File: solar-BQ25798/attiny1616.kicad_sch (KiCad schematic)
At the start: 14 parts, among them J1901 Conn_01x04, U1901 ATtiny1616-M

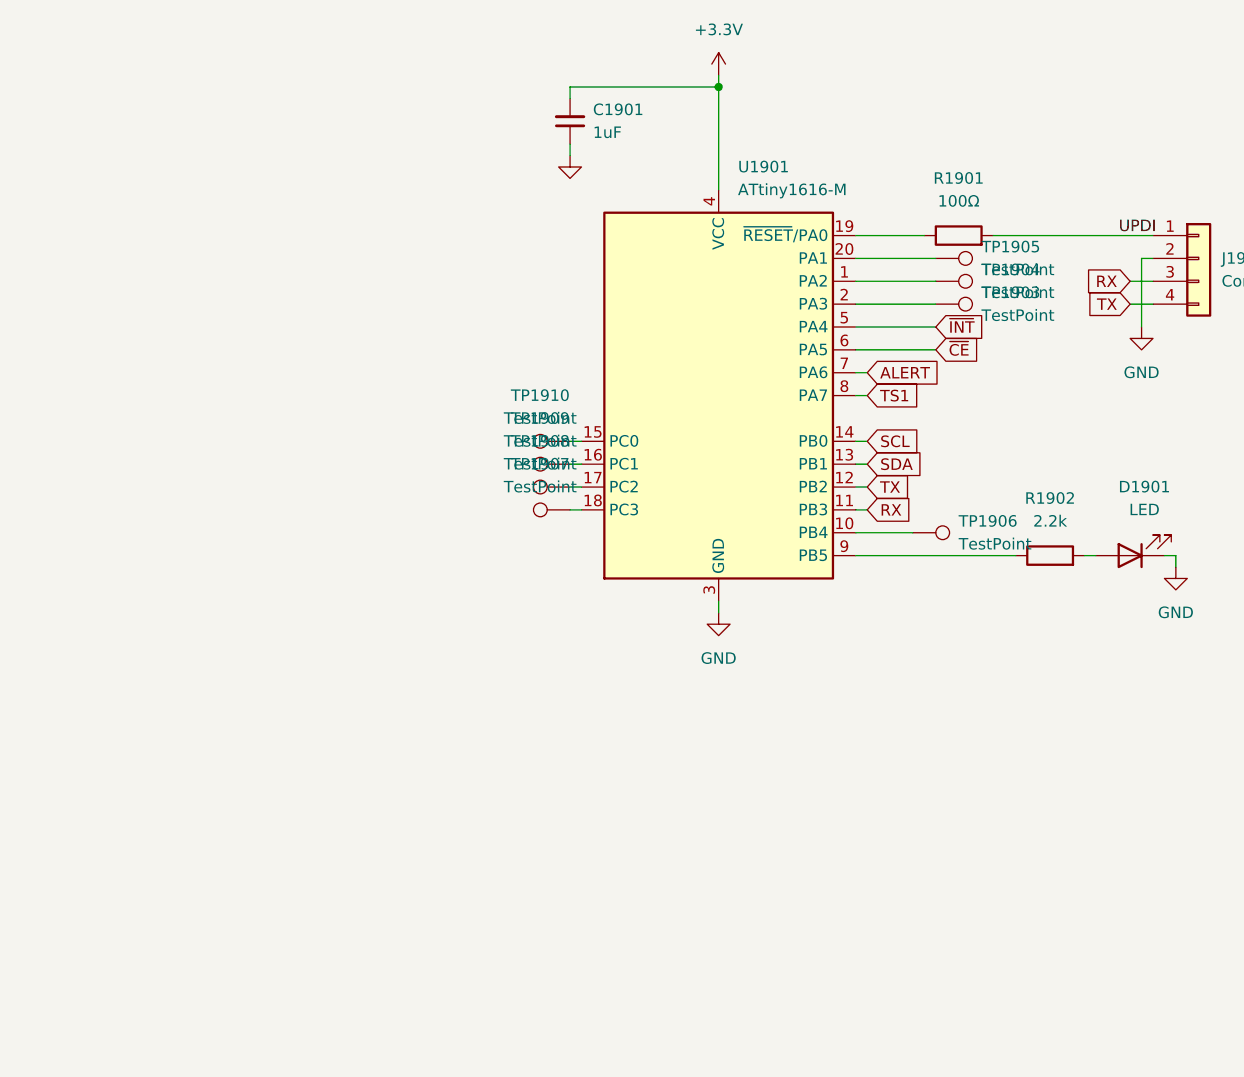
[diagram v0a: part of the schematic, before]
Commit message: BQ25798 WIP
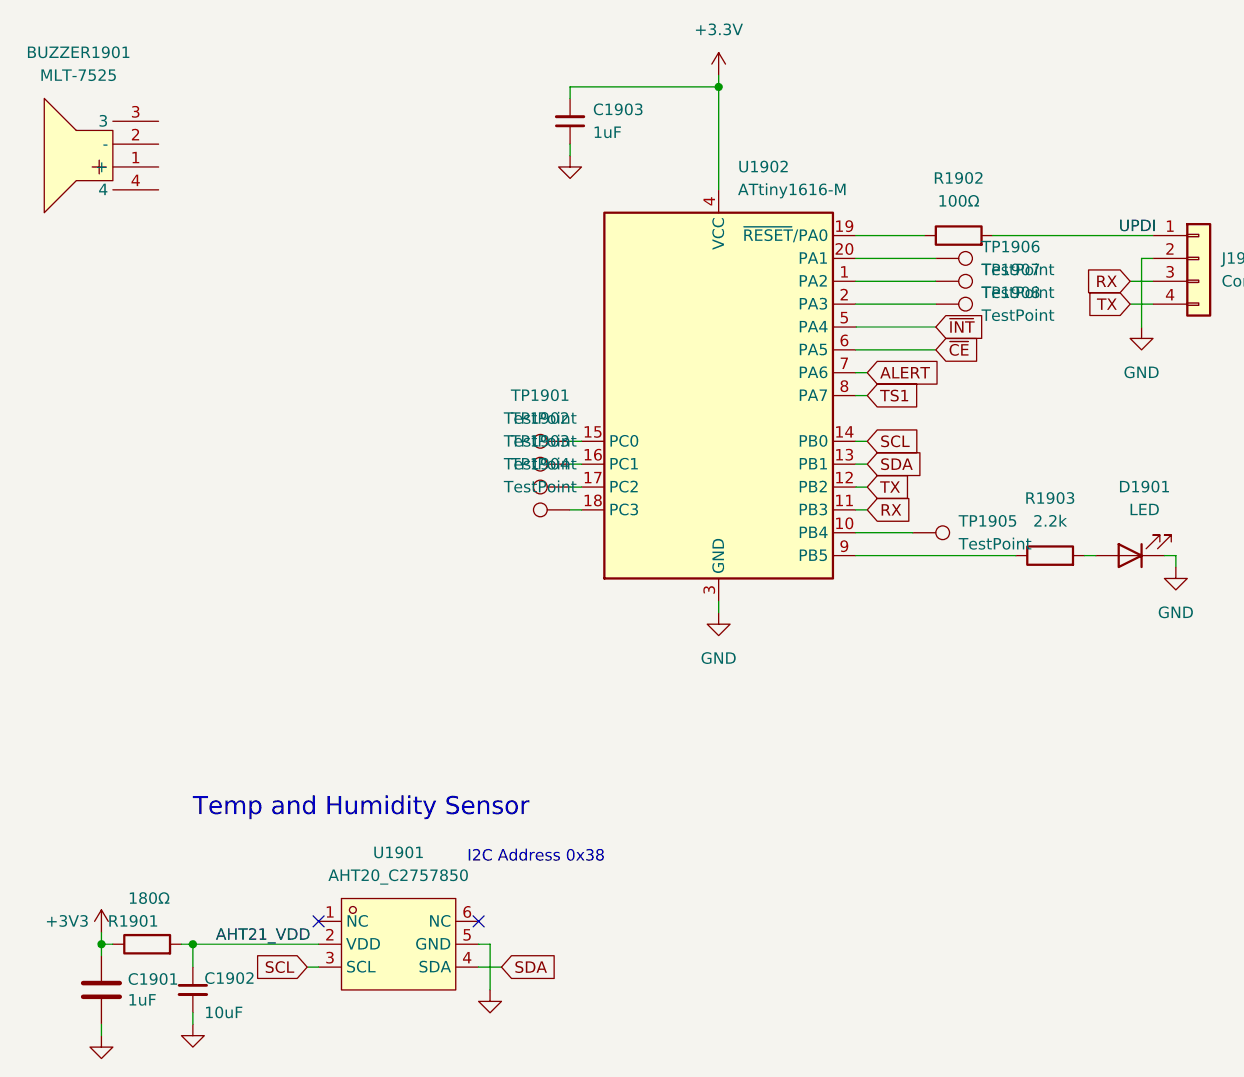
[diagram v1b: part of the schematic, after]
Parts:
- added BUZZER1901: MLT-7525, cacophony-library:BUZ-SMD_4P-L7.5-W7.5-P7.59-TL, symbol cacophony-library:MLT-7525
- added C1901: 1uF, Capacitor_SMD:C_0402_1005Metric, symbol Device:C
- added C1902: 10uF, Capacitor_SMD:C_0603_1608Metric, symbol Device:C_Small
- added R1901: 180Ω, Resistor_SMD:R_0402_1005Metric, symbol Device:R
- added U1901: AHT20_C2757850, cacophony-library:SENSOR-SMD_L3.0-W3.0-P1.00-BR, symbol cacophony-library:AHT20_C2757850
- renumbered C1901 to C1903, R1901 to R1902, R1902 to R1903, TP1910 to TP1901, TP1909 to TP1902, TP1908 to TP1903, TP1907 to TP1904, TP1906 to TP1905, TP1905 to TP1906, TP1904 to TP1907, TP1903 to TP1908, U1901 to U1902
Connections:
- net GND: now also C1901.2, C1902.2, U1901.5 (GND)
- net SCL: now also U1901.3 (SCL)
- net SDA: now also U1901.4 (SDA)
- new net +3V3: C1901.1, R1901.1
- new net AHT21_VDD: C1902.1, R1901.2, U1901.2 (VDD)
- no-connect marks 0 -> 2
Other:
- note added: "I2C Address 0x38"
- note added: "Temp and Humidity Sensor"

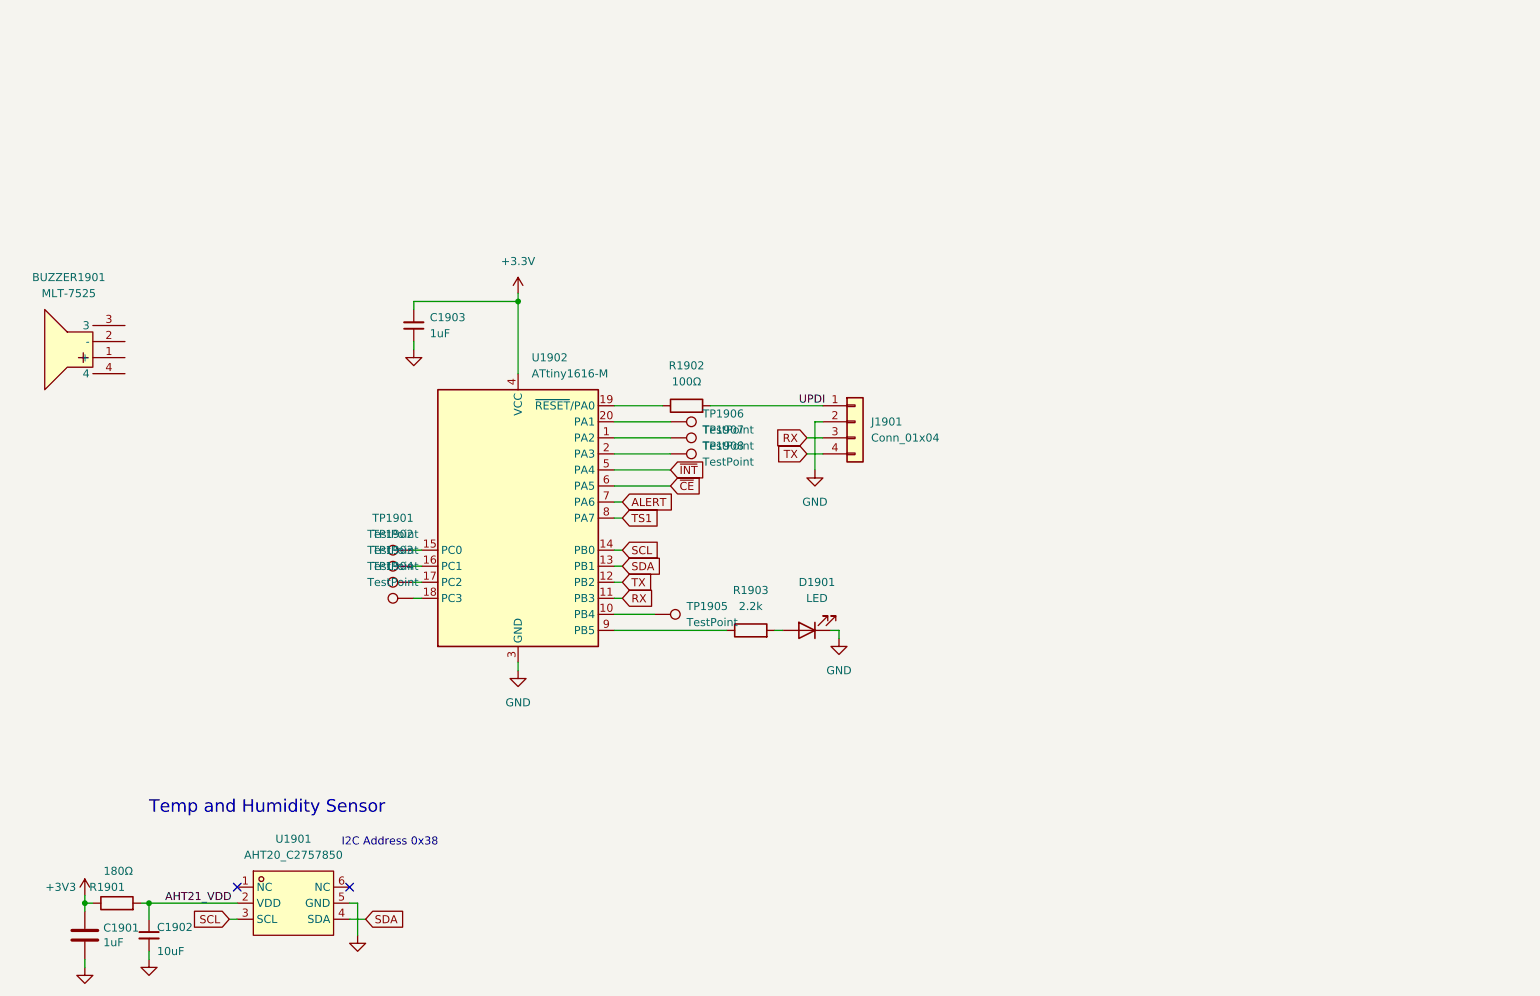
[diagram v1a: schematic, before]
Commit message: Solar battery WIP
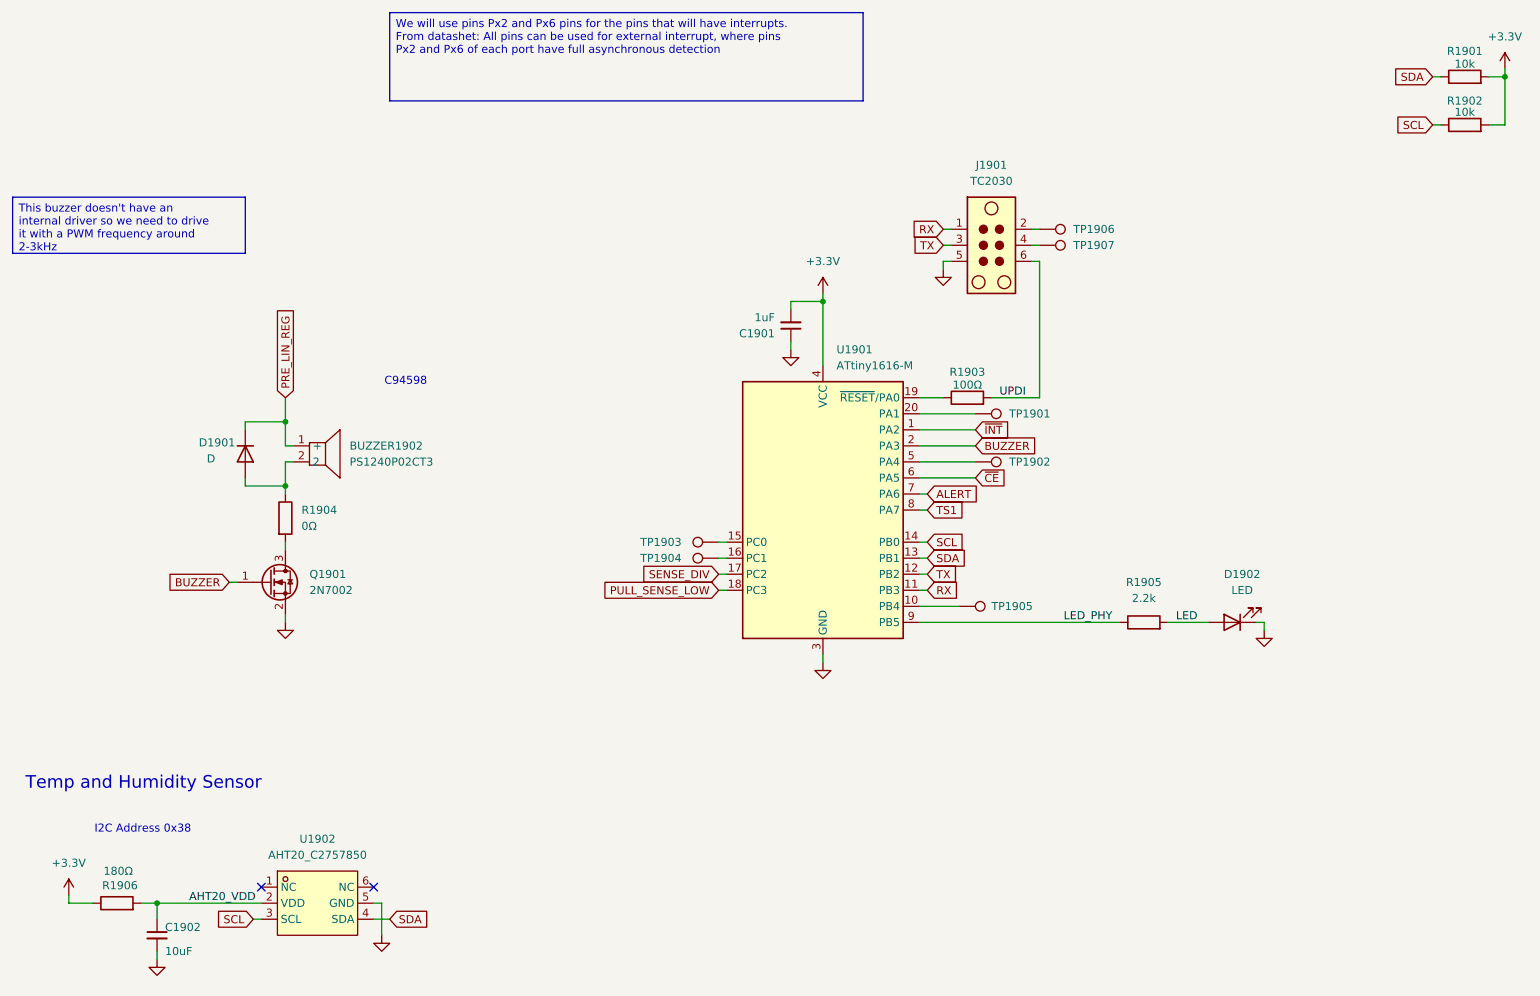
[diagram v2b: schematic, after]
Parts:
- removed BUZZER1901: MLT-7525, cacophony-library:BUZ-SMD_4P-L7.5-W7.5-P7.59-TL, symbol cacophony-library:MLT-7525
- removed C1901: 1uF, Capacitor_SMD:C_0402_1005Metric, symbol Device:C
- removed J1901: Conn_01x04, Connector_PinHeader_2.00mm:PinHeader_1x04_P2.00mm_Vertical, symbol Connector_Generic:Conn_01x04
- removed TP1903, TP1904, TP1908: TestPoint, cacophony-library:TP_PAD, symbol cacophony-library:TestPoint
- added BUZZER1902: PS1240P02CT3, cacophony-library:BUZ-TH_BD12.5-P5.00-D0.9, symbol cacophony-library:PS1240P02CT3
- added D1901: D, Diode_SMD:D_SOD-323_HandSoldering, symbol Device:D
- added J1901: TC2030, Connector:Tag-Connect_TC2030-IDC-NL_2x03_P1.27mm_Vertical, symbol Connector:TC2030
- added Q1901: 2N7002, Package_TO_SOT_SMD:SOT-23, symbol Transistor_FET:2N7002
- added R1901, R1902: 10k, Resistor_SMD:R_0402_1005Metric, symbol Device:R
- added R1904: 0Ω, Resistor_SMD:R_0805_2012Metric, symbol Device:R
- added TP1906, TP1907: TestPoint, cacophony-library:TP_PAD, symbol cacophony-library:TestPoint
- renumbered C1903 to C1901, D1901 to D1902, R1902 to R1903, R1903 to R1905, R1901 to R1906, TP1906 to TP1901, TP1907 to TP1902, TP1901 to TP1903, TP1902 to TP1904, U1902 to U1901, U1901 to U1902
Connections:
- net +3V3 is gone; now on net +3.3V: R1906.1
- net +3.3V: now also R1901.2, R1902.2
- net GND: now also J1901.5, Q1901.2 (S)
- net RX: now also J1901.1
- net SCL: now also R1902.1
- net SDA: now also R1901.1
- net TX: now also J1901.3
- net UPDI: now also J1901.6
- net ~{INT}: now also U1901.1 (PA2); no longer U1901.5 (PA4)
- net LED_PHY: now reaches R1905.1, U1901.9 (PB5)
- net LED: now reaches D1902.2 (A), R1905.2
- net PULL_SENSE_LOW: now reaches U1901.18 (PC3)
- net BUZZER: now reaches U1901.2 (PA3)
- net BUZZER: now also Q1901.1 (G)
- net at TP1902.1: now also U1901.5 (PA4); no longer U1901.1 (PA2)
- net SENSE_DIV: now reaches U1901.17 (PC2)
- net AHT21_VDD renamed AHT20_VDD
- new net: BUZZER1902.2, D1901.2 (A), R1904.1
- new net: Q1901.3 (D), R1904.2
- new net: J1901.2, TP1906.1
- new net: J1901.4, TP1907.1
- new net PRE_LIN_REG: BUZZER1902.1 (+), D1901.1 (K)
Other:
- note added: "C94598"
- moved on the sheet: C1901, C1902, D1902, R1903, R1905, TP1901, TP1902, TP1903, TP1904, TP1905, U1901, U1902

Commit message: Version v0.0.2
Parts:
- D1901: LCSC Part (none) -> C2128
- Q1901: LCSC Part (none) -> C8545
- R1904: LCSC Part (none) -> C17477
- U1901: LCSC Part (none) -> C507118
- U1902: LCSC Part C2757850 -> C3012622
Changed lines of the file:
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@@
+			)
+		)
+		(property "LCSC Part" "C17477"
+			(at 71.12 102.87 0)
+			(effects
+				(font
+					(size 1.27 1.27)
+				)
+				(hide yes)
 			)
 		)
@@
 			)
 		)
+		(property "LCSC Part" "C8545"
+			(at 68.58 113.03 0)
+			(effects
+				(font
+					(size 1.27 1.27)
+				)
+				(hide yes)
+			)
+		)
 		(pin "1"
 		)
@@
 			)
 		)
+		(property "LCSC Part" "C2128"
+			(at 64.77 92.71 90)
+			(effects
+				(font
+					(size 1.27 1.27)
+				)
+				(hide yes)
+			)
+		)
 		(pin "2"
 		)
@@
 			)
 		)
+		(property "LCSC Part" "C507118"
+			(at 156.21 101.6 0)
+			(effects
+				(font
+					(size 1.27 1.27)
+				)
+				(hide yes)
+			)
+		)
 		(pin "1"
 		)
@@
 			)
 		)
-		(property "LCSC Part" "C2757850"
+		(property "LCSC Part" "C3012622"
 			(at 76.2 163.83 0)
 			(effects
